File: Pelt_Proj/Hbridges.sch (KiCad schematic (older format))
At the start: 24 parts

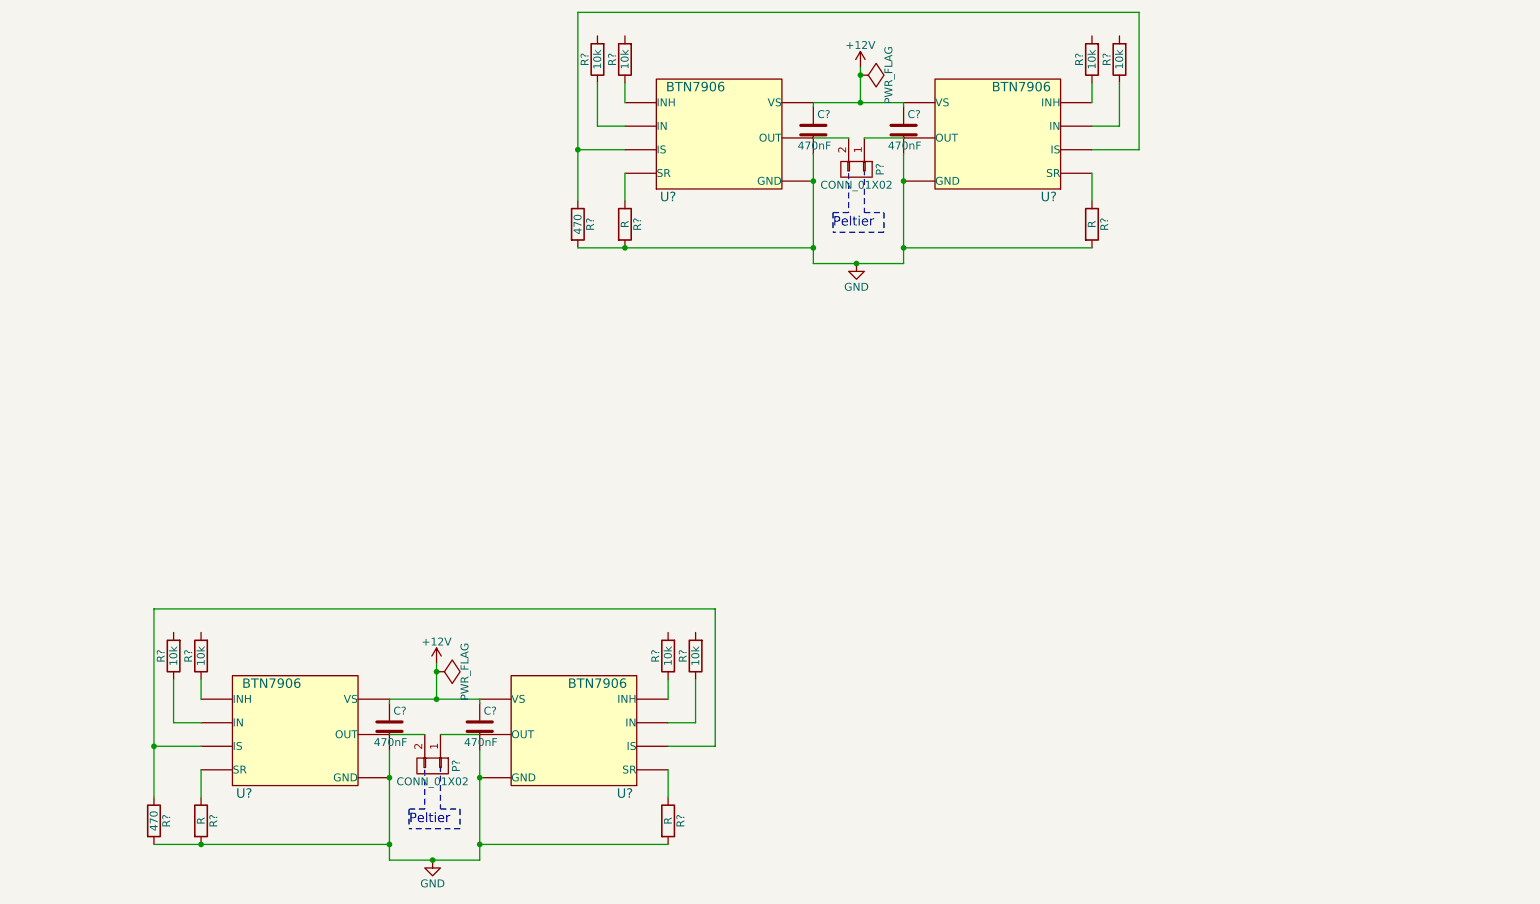
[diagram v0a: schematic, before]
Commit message: with new hbridge file
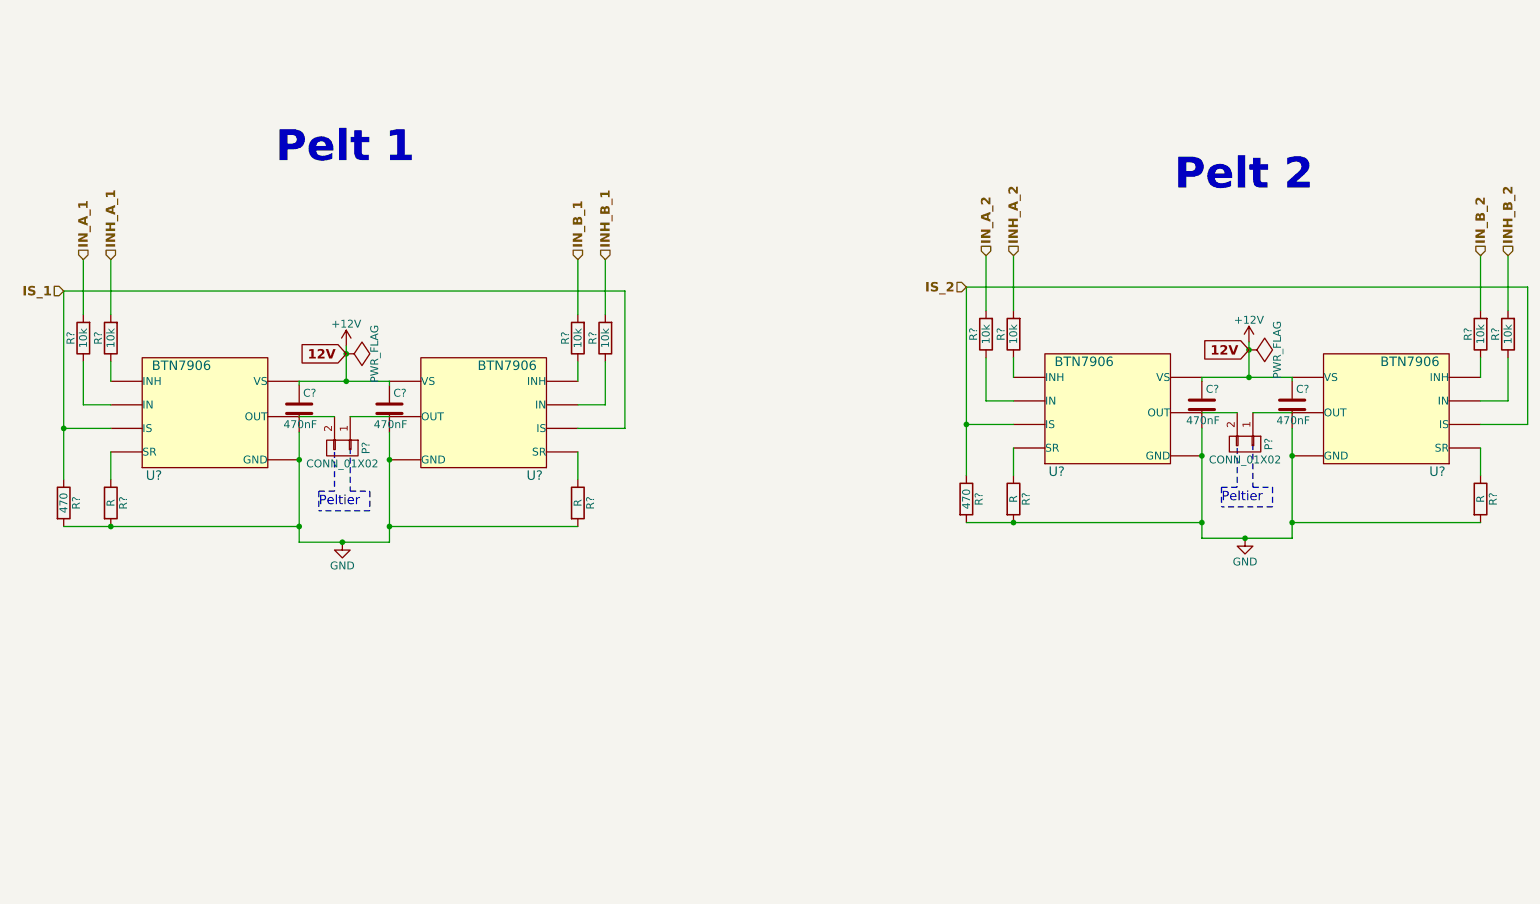
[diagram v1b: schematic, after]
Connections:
- net INH_A_1: now reaches R?.2
- net IS_1: now reaches R?.1, U?.6 (IS), U?.6 (IS)
- net IN_A_1: now reaches R?.2
- net IN_B_1: now reaches R?.2
- net INH_B_1: now reaches R?.2
- net INH_A_2: now reaches R?.2
- net IS_2: now reaches R?.1, U?.6 (IS), U?.6 (IS)
- net IN_A_2: now reaches R?.2
- net IN_B_2: now reaches R?.2
- net INH_B_2: now reaches R?.2
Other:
- note added: "Pelt 1"
- note added: "Pelt 2"
- moved on the sheet: C?, P?, R?, U?
